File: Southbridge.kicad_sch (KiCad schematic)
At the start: 36 parts, among them J1 SM03B-SRSS-TB, J2 SM03B-SRSS-TB, J3 USB_C_Receptacle_USB2.0_16P, SW1 SW_Push, SW2 SW_Push, U1 USBLC6-2SC6, U2 RP2350_80QFN, U3 W25Q16JVSS, Y1 ABM8-272-T3

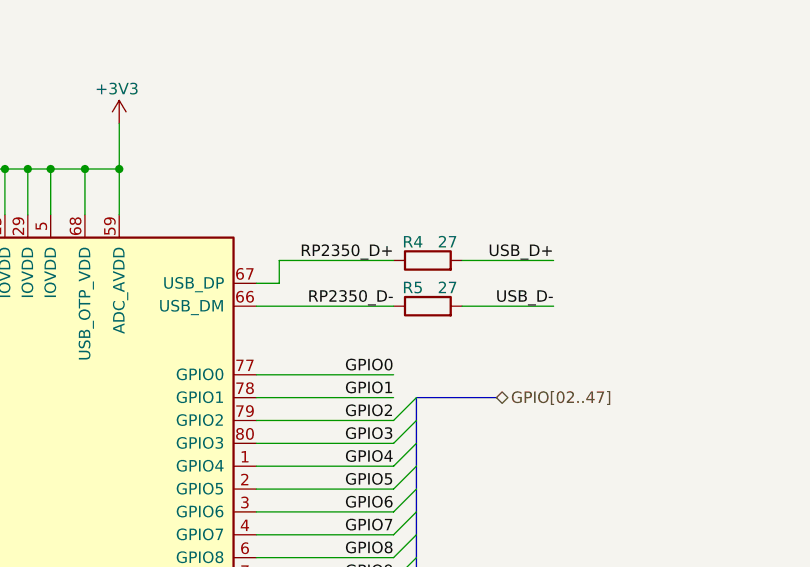
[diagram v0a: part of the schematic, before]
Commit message: V2.0.0 WIP
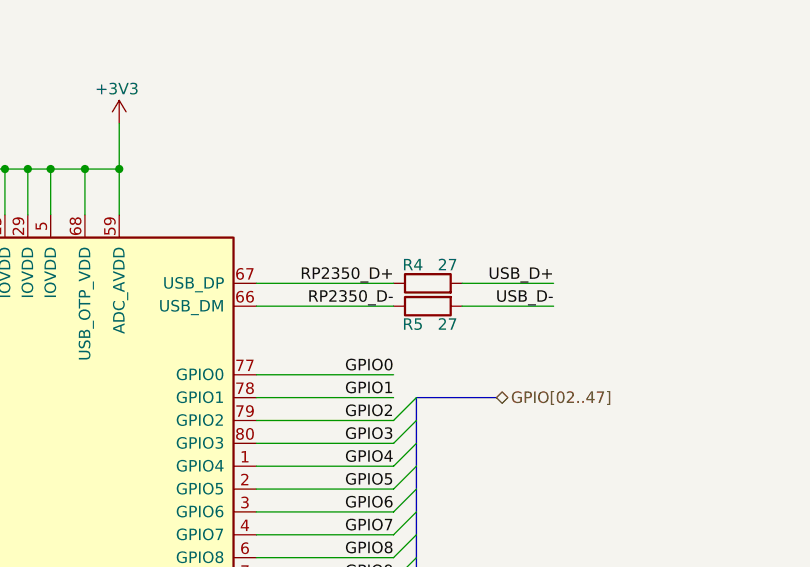
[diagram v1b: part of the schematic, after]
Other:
- moved on the sheet: R4
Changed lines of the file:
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@@
 	(wire
 		(pts
-			(xy 160.02 134.62) (xy 160.02 137.16)
-		)
-		(stroke
-			(width 0)
-			(type default)
-		)
-	)
-	(wire
-		(pts
 			(xy 157.48 210.82) (xy 172.72 210.82)
 		)
@@
 	(wire
 		(pts
-			(xy 190.5 134.62) (xy 180.34 134.62)
+			(xy 190.5 137.16) (xy 180.34 137.16)
 		)
 		(stroke
@@
 	(wire
 		(pts
-			(xy 160.02 134.62) (xy 172.72 134.62)
-		)
-		(stroke
-			(width 0)
-			(type default)
-		)
-	)
-	(wire
-		(pts
 			(xy 157.48 139.7) (xy 172.72 139.7)
 		)
@@
 	(wire
 		(pts
-			(xy 160.02 137.16) (xy 157.48 137.16)
+			(xy 157.48 137.16) (xy 172.72 137.16)
 		)
 		(stroke
@@
 	)
 	(label "USB_D+"
-		(at 190.5 134.62 180)
+		(at 190.5 137.16 180)
 		(effects
 			(font
@@
 	)
 	(label "RP2350_D+"
-		(at 172.72 134.62 180)
+		(at 172.72 137.16 180)
 		(effects
 			(font
@@
 		(lib_id "Device:R")
 		(at 176.53 139.7 90)
+		(mirror x)
 		(unit 1)
 		(exclude_from_sim no)
@@
 		(dnp no)
 		(property "Reference" "R5"
-			(at 176.022 137.668 90)
+			(at 176.022 141.732 90)
 			(effects
 				(font
@@
 		)
 		(property "Value" "27"
-			(at 179.832 137.668 90)
+			(at 179.832 141.732 90)
 			(effects
 				(font
@@
 		)
 		(property "Footprint" "Resistor_SMD:R_0402_1005Metric_Pad0.72x0.64mm_HandSolder"
-			(at 176.53 141.478 90)
+			(at 176.53 137.922 90)
 			(effects
 				(font
@@
 	(symbol
 		(lib_id "Device:R")
-		(at 176.53 134.62 90)
+		(at 176.53 137.16 90)
 		(unit 1)
 		(exclude_from_sim no)
@@
 		(dnp no)
 		(property "Reference" "R4"
-			(at 176.022 132.588 90)
+			(at 176.022 135.128 90)
 			(effects
 				(font
@@
 		)
 		(property "Value" "27"
-			(at 179.832 132.588 90)
+			(at 179.832 135.128 90)
 			(effects
 				(font
@@
 		)
 		(property "Footprint" "Resistor_SMD:R_0402_1005Metric_Pad0.72x0.64mm_HandSolder"
-			(at 176.53 136.398 90)
+			(at 176.53 138.938 90)
 			(effects
 				(font
@@
 		)
 		(property "Datasheet" "~"
-			(at 176.53 134.62 0)
+			(at 176.53 137.16 0)
 			(effects
 				(font
@@
 		)
 		(property "Description" "Resistor"
-			(at 176.53 134.62 0)
+			(at 176.53 137.16 0)
 			(effects
 				(font

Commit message: Update BOM
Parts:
- R1, R2: now left out of the parts list
- R6, R7, R8: now in the parts list
- U2: LCSC PN (none) -> C42415655
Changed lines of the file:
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@@
 		(unit 1)
 		(exclude_from_sim no)
-		(in_bom yes)
+		(in_bom no)
 		(on_board yes)
 		(dnp no)
@@
 			)
 		)
+		(property "LCSC PN" "C42415655"
+			(at 120.65 180.34 0)
+			(effects
+				(font
+					(size 1.27 1.27)
+				)
+				(hide yes)
+			)
+		)
 		(pin "1"
 		)
@@
 		(unit 1)
 		(exclude_from_sim no)
-		(in_bom no)
+		(in_bom yes)
 		(on_board yes)
 		(dnp no)
@@
 		(unit 1)
 		(exclude_from_sim no)
-		(in_bom no)
+		(in_bom yes)
 		(on_board yes)
 		(dnp no)
@@
 		(unit 1)
 		(exclude_from_sim no)
-		(in_bom yes)
+		(in_bom no)
 		(on_board yes)
 		(dnp no)
@@
 		(unit 1)
 		(exclude_from_sim no)
-		(in_bom no)
+		(in_bom yes)
 		(on_board yes)
 		(dnp no)
